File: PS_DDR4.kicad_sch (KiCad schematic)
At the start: 2 parts, among them U12 K4A8G165WC-BCTD

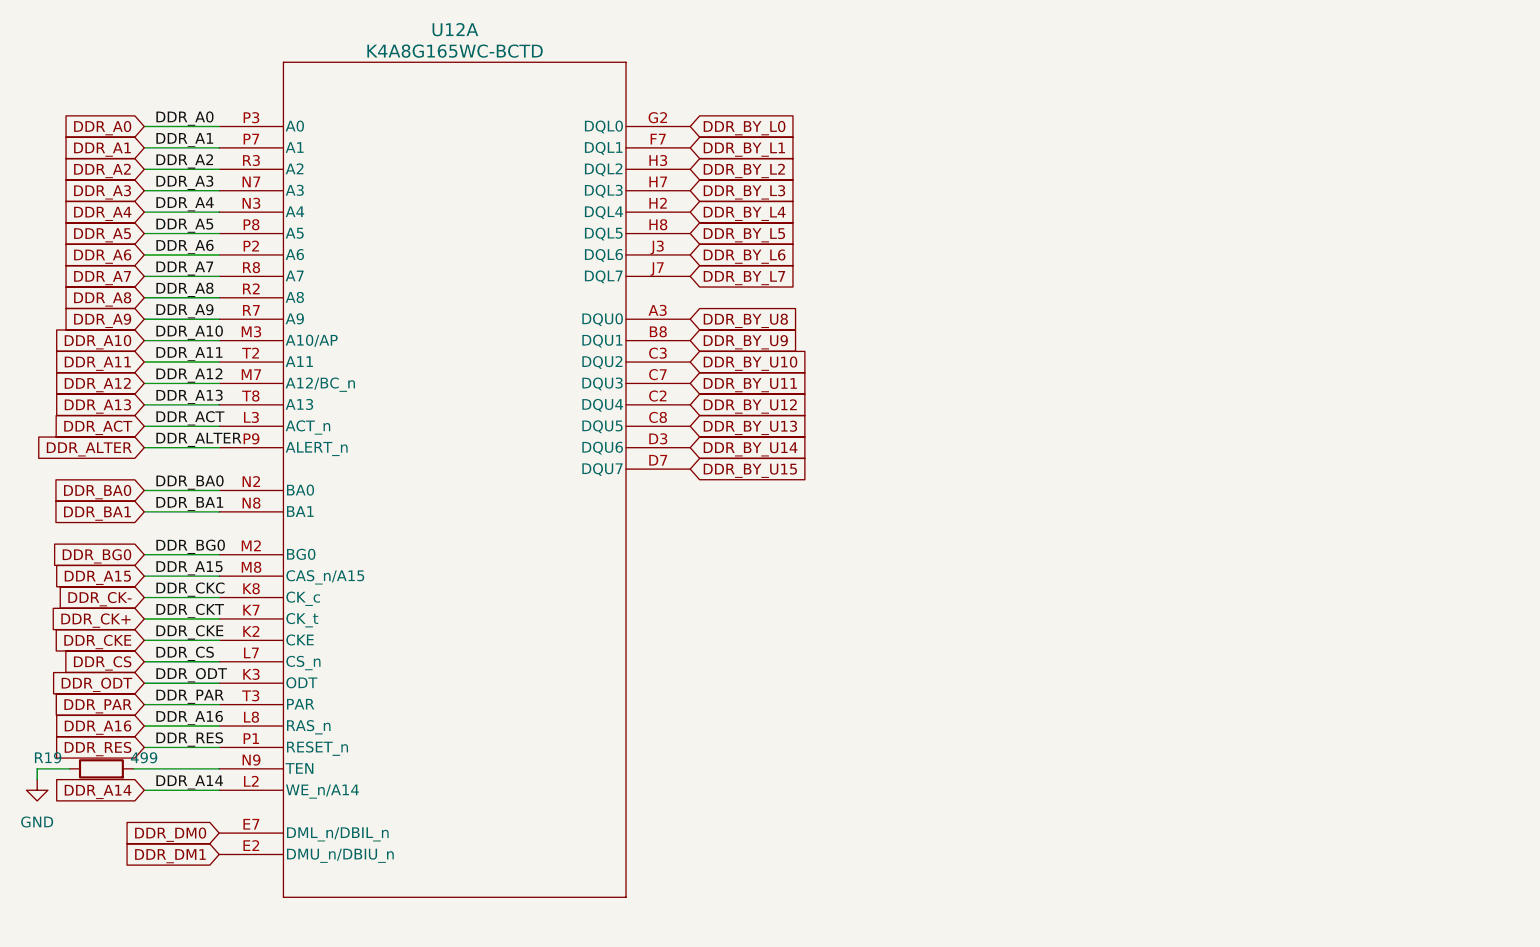
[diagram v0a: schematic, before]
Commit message: Stuff
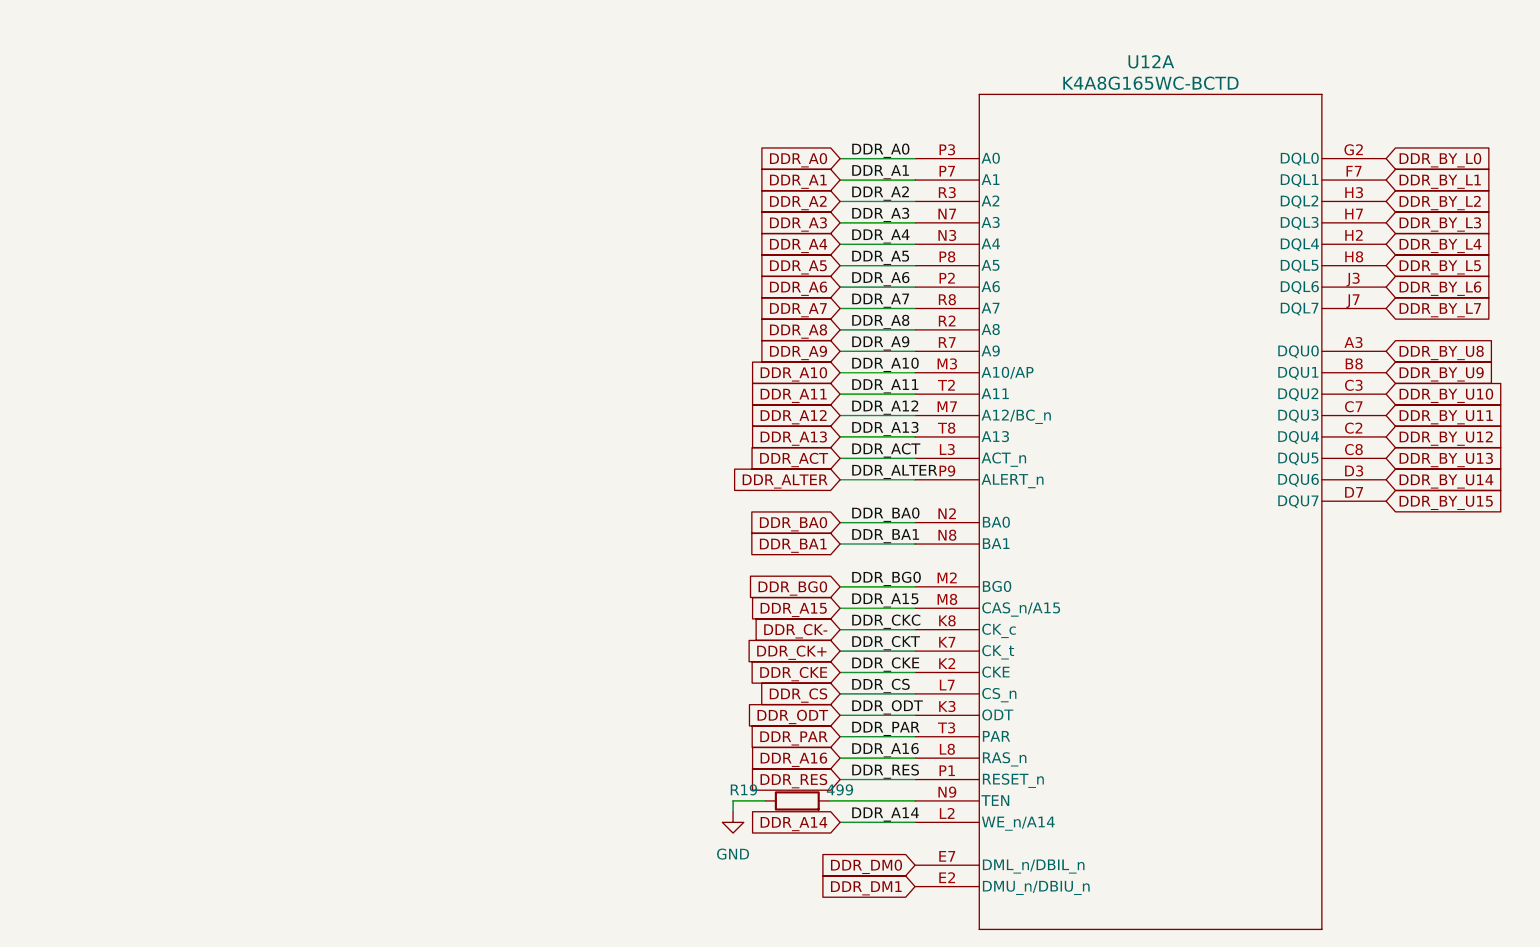
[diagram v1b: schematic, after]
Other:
- moved on the sheet: R19, U12A
